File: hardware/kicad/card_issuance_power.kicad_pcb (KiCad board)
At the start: 2 copper layers, 124.5 x 132.5 mm, 39 parts, among them J1 V12_IN, J2 V12_OUT, J3 V3V3_OUT, J4 V5.1_OUT, Q1 IRF4905, U1 PTSM82903SISB2R, U2 LMZ23610TZ/NOPB

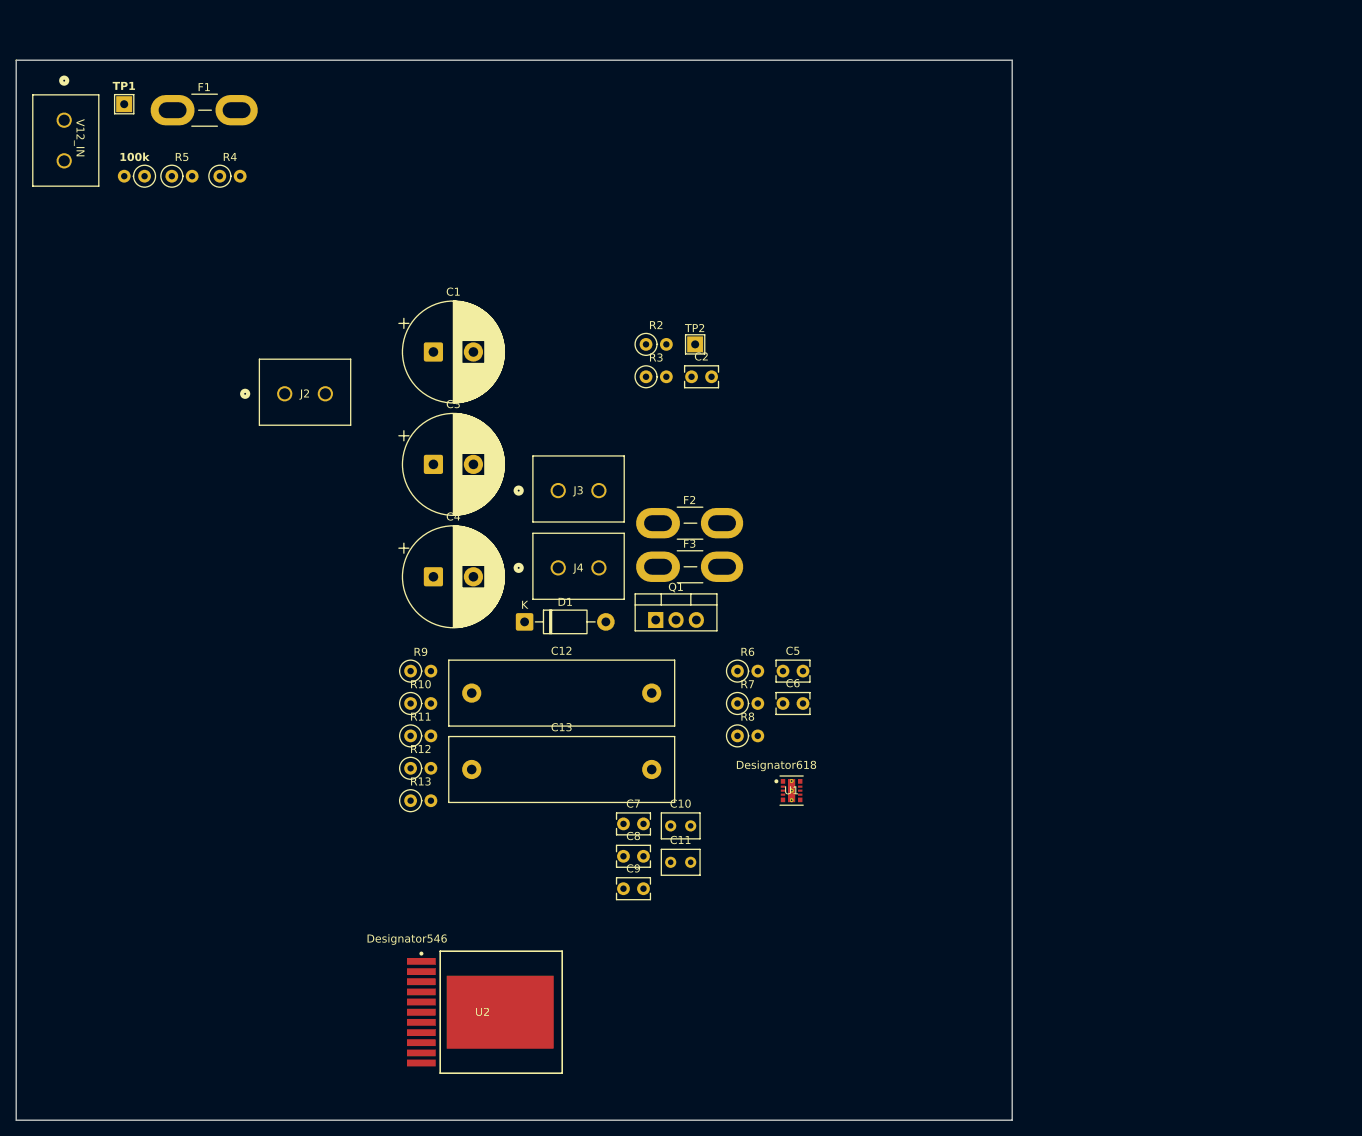
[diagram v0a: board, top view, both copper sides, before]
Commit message: feat: added settings - pcb design
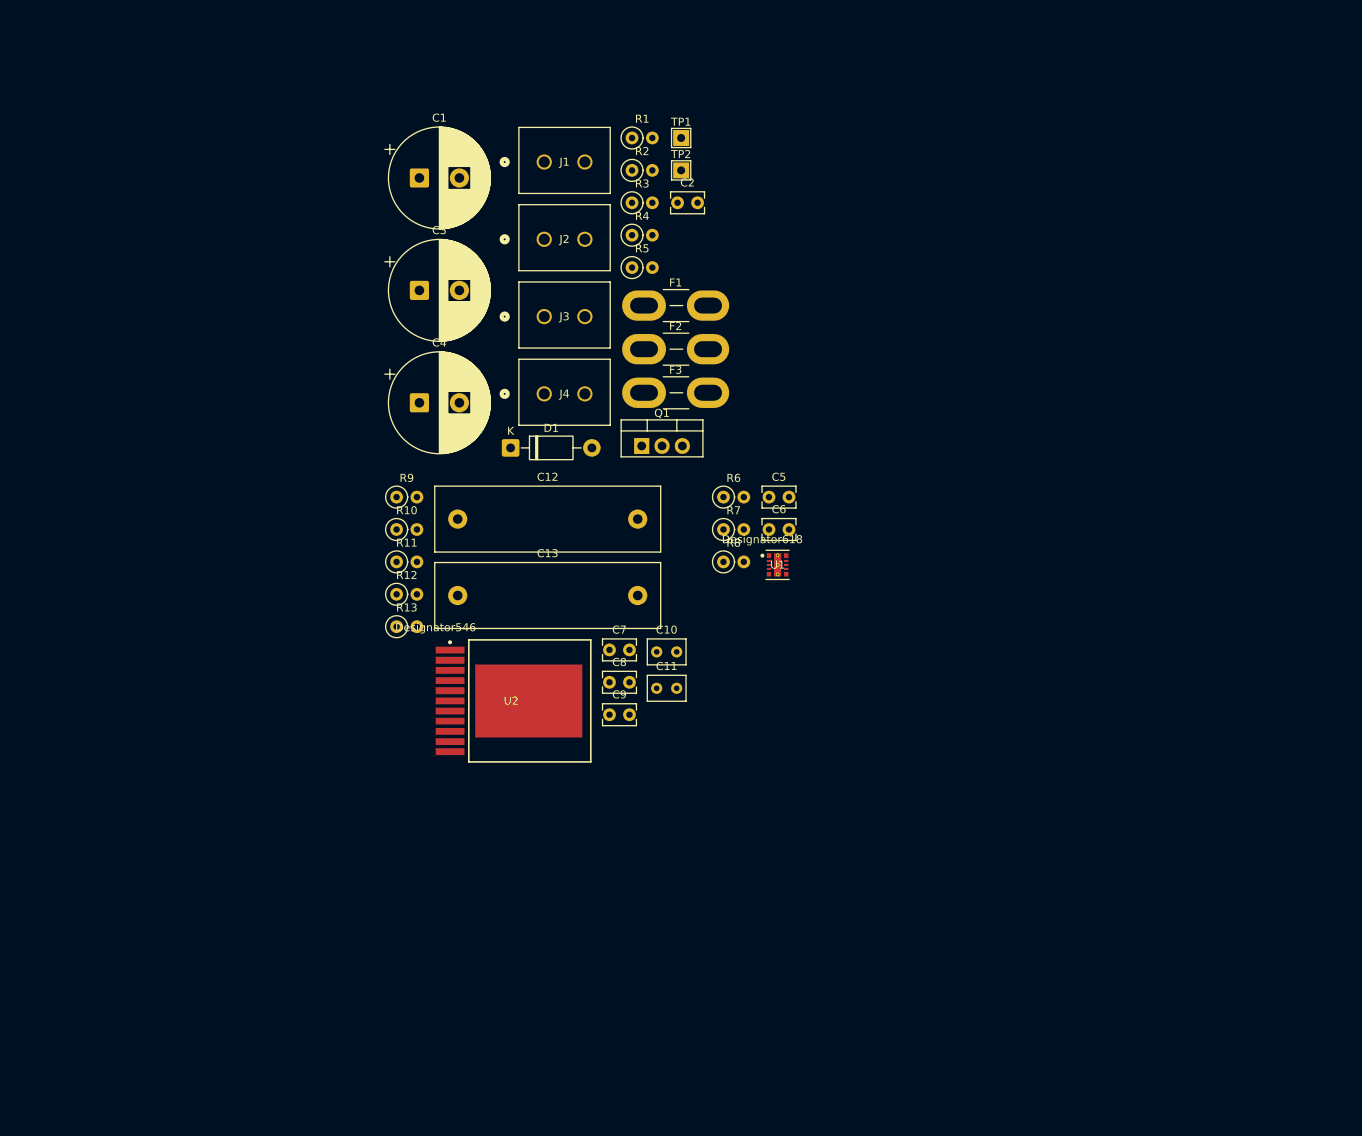
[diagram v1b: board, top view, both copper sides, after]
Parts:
- moved TP1 69.7 mm to (128.6, 34.2)
- moved F1 63.8 mm to (124.0, 55.2)
- moved R1 61.1 mm to (122.5, 34.2), turned to 0 degrees
- moved J1 60.2 mm to (111.5, 37.2), turned to 0 degrees
- moved R5 58.6 mm to (122.5, 50.4)
- moved R4 52.0 mm to (122.5, 46.4)
- moved U2 39.1 mm to (107.4, 104.6)
- moved J2 37.8 mm to (111.5, 46.9)
- moved U1 28.3 mm to (140.7, 87.6)
- moved C2 21.8 mm to (128.2, 42.3)
- moved R3 21.8 mm to (122.5, 42.3)
- moved C1 21.8 mm to (95.9, 39.2)
- moved C10 21.8 mm to (125.6, 98.5)
- moved C11 21.8 mm to (125.6, 103.0)
- moved C12 21.8 mm to (100.7, 81.9)
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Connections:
- net /BUCK_3V3/VIN renamed /V12_PROT_5V
- net /BUCK_3V3/VOUT renamed /V3V3_OUT
- net /BUCK_5.1/VOUT renamed /V5.1_OUT
- net Net-(D1-A) renamed /V12_FUSED
- net Net-(J1-Pin_1) renamed /V12_IN
- net Net-(J1-Pin_2) renamed /GND_STAR
- net Net-(J2-Pin_1) renamed /V12_PROT_12V
- net Net-(Q1-D) renamed /V12_PROT
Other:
- board outline removed
- copper layers 2 -> 4

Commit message: chore: pcb board components placements
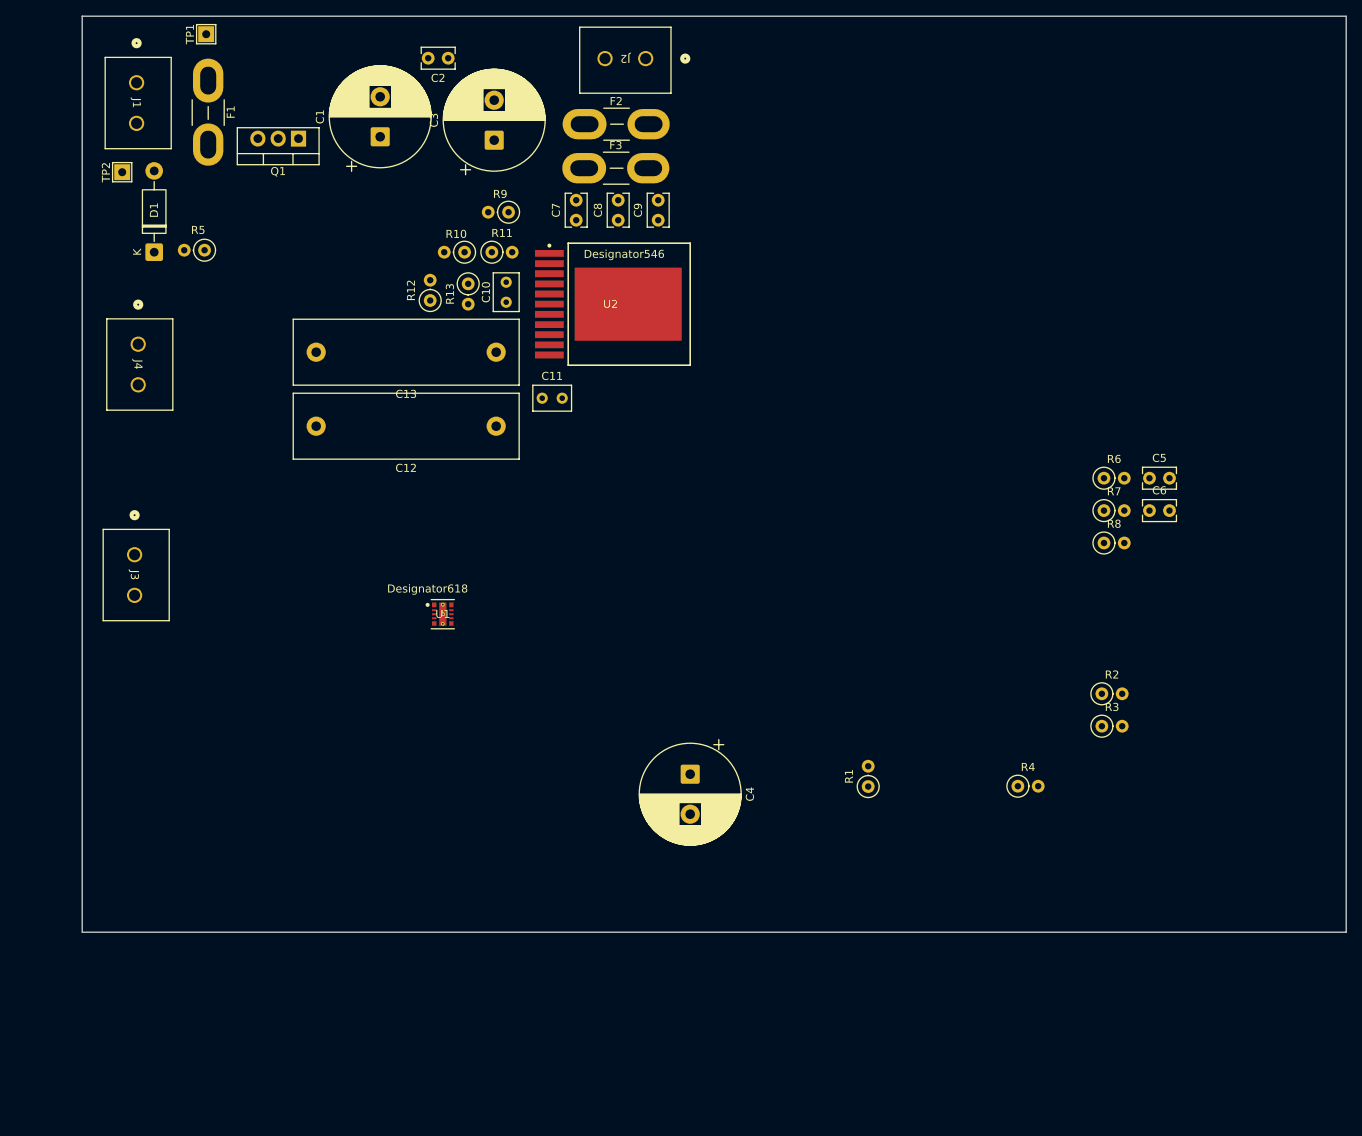
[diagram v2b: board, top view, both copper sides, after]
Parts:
- moved R2 87.9 mm to (181.2, 103.7)
- moved R3 87.9 mm to (181.2, 107.8)
- moved R1 86.3 mm to (152.0, 115.3), turned to 90 degrees
- moved R4 84.1 mm to (170.7, 115.2)
- moved TP2 69.9 mm to (58.8, 38.5), turned to 90 degrees
- moved C9 62.1 mm to (125.8, 44.5), turned to 90 degrees
- moved F1 61.3 mm to (69.5, 27.1), turned to -90 degrees
- moved TP1 60.8 mm to (69.2, 21.2), turned to 90 degrees
- moved J3 59.2 mm to (60.3, 86.3), turned to -90 degrees
- moved C8 57.8 mm to (120.8, 44.5), turned to 90 degrees
- moved Q1 57.6 mm to (80.8, 34.3), turned to 180 degrees
- moved C4 57.5 mm to (129.8, 113.8), turned to -90 degrees
- moved C7 53.9 mm to (115.5, 44.5), turned to 90 degrees
- moved R5 53.5 mm to (69.0, 48.2), turned to 180 degrees
- moved J1 51.9 mm to (60.6, 27.3), turned to -90 degrees
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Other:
- board outline added: 158 x 114.5 mm
